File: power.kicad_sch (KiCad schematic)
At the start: 19 parts, among them J9 DC Barrel Jack, U2 LMR33620CQ5, U3 TLV76733

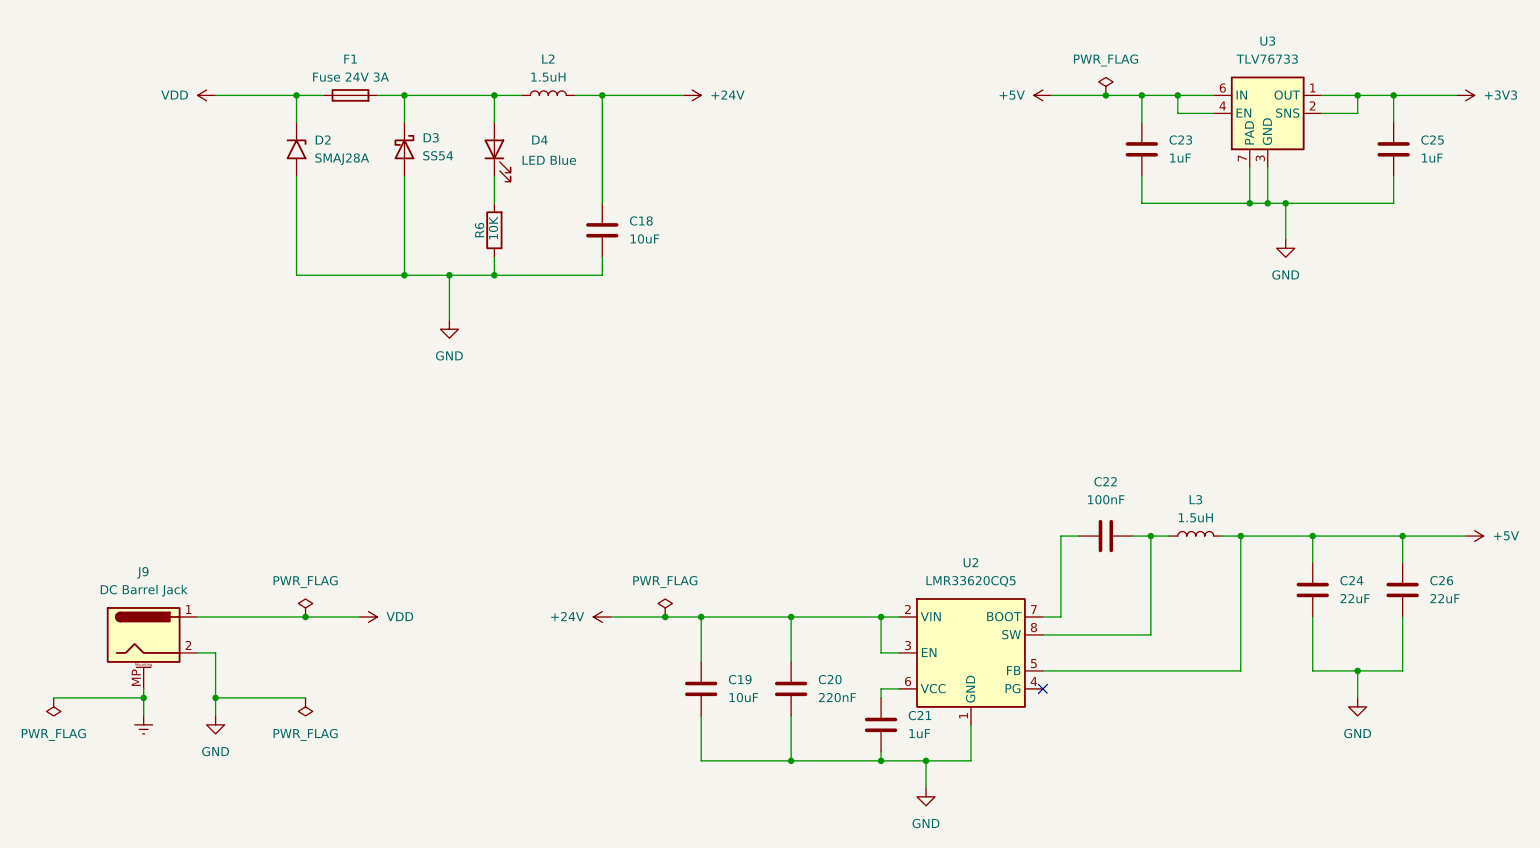
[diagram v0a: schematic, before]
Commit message: Excluded rare components
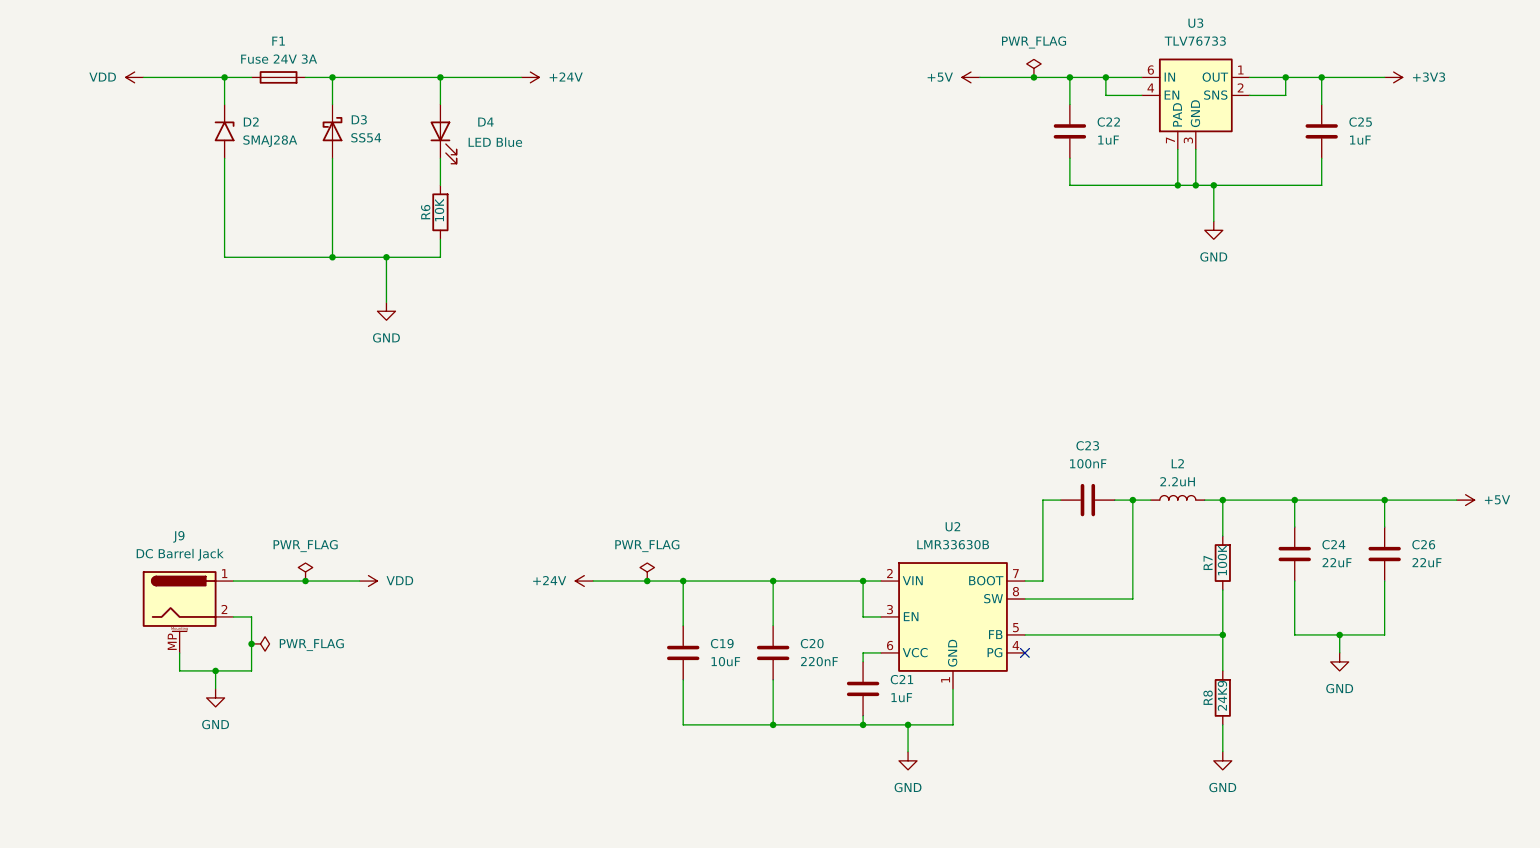
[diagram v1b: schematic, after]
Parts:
- removed C18: 10uF, Capacitor_SMD:C_1206_3216Metric_Pad1.33x1.80mm_HandSolder, symbol Device:C
- removed L2: 1.5uH, Inductor_SMD:L_Bourns_SRP5030T, symbol Device:L
- removed U2: LMR33620CQ5, Package_SO:Texas_HSOP-8-1EP_3.9x4.9mm_P1.27mm_ThermalVias, symbol Regulator_Switching:LMR33620ADDA
- added R7: 100K, Resistor_SMD:R_0603_1608Metric_Pad0.98x0.95mm_HandSolder, symbol Device:R
- added R8: 24K9, Resistor_SMD:R_0603_1608Metric_Pad0.98x0.95mm_HandSolder, symbol Device:R
- added U2: LMR33630B, Package_SO:Texas_HSOP-8-1EP_3.9x4.9mm_P1.27mm_ThermalVias, symbol Regulator_Switching:LMR33630ADDA
- L2: renamed from L3; value 1.5uH -> 2.2uH; footprint Inductor_SMD:L_Bourns_SRP5030T -> Inductor_SMD:L_10.4x10.4_H4.8
- renumbered C23 to C22, C22 to C23
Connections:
- net Earth is gone; now on net GND: J9.MP (MountPin)
- net +24V: now also D3.1 (K), D4.2 (A), F1.2, U2.2 (VIN), U2.3 (EN)
- net +5V: now also R7.2
- net GND: now also R8.1, U2.1 (GND), U2.9 (GND)
- net at C21.1: now also U2.6 (VCC)
- net at C23.1: now also U2.7 (BOOT)
- net at C23.2, L2.1: now also U2.8 (SW)
- new net: R7.1, R8.2, U2.5 (FB)
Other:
- moved on the sheet: C19, C20, C21, C22, C23, C24, C25, C26, D2, D3, D4, F1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
